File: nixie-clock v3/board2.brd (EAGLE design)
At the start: 158.4 x 50.2 mm, 15 parts

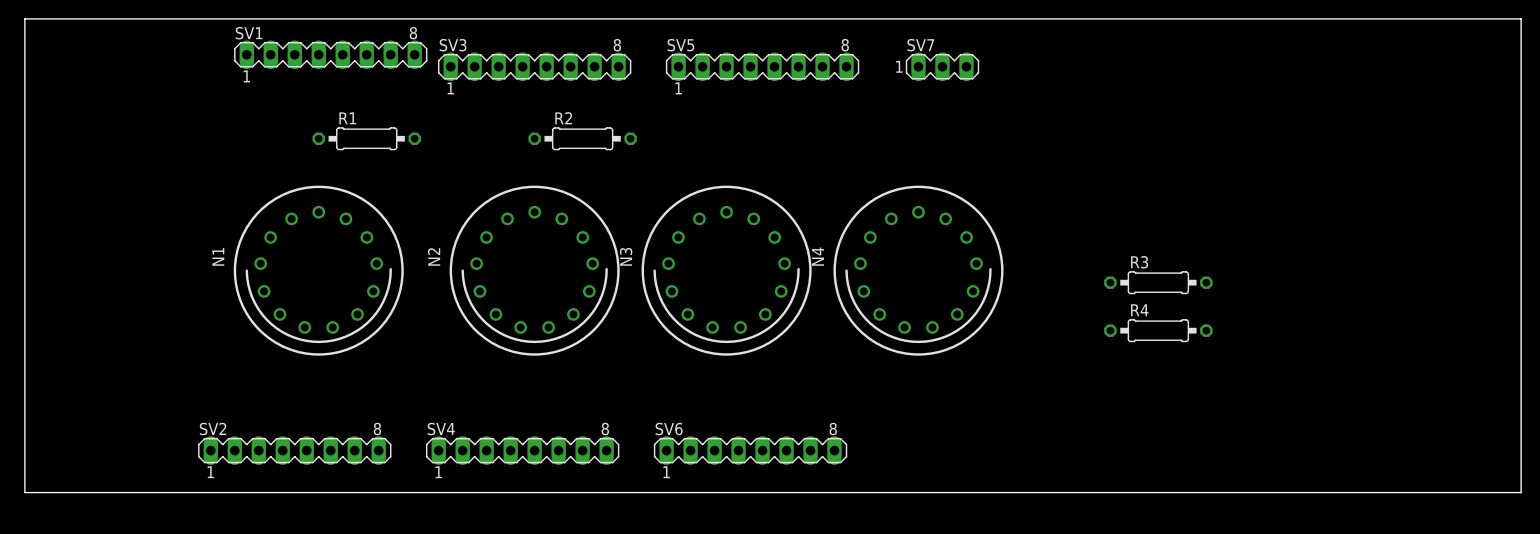
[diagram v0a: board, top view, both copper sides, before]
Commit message: lots of board progress
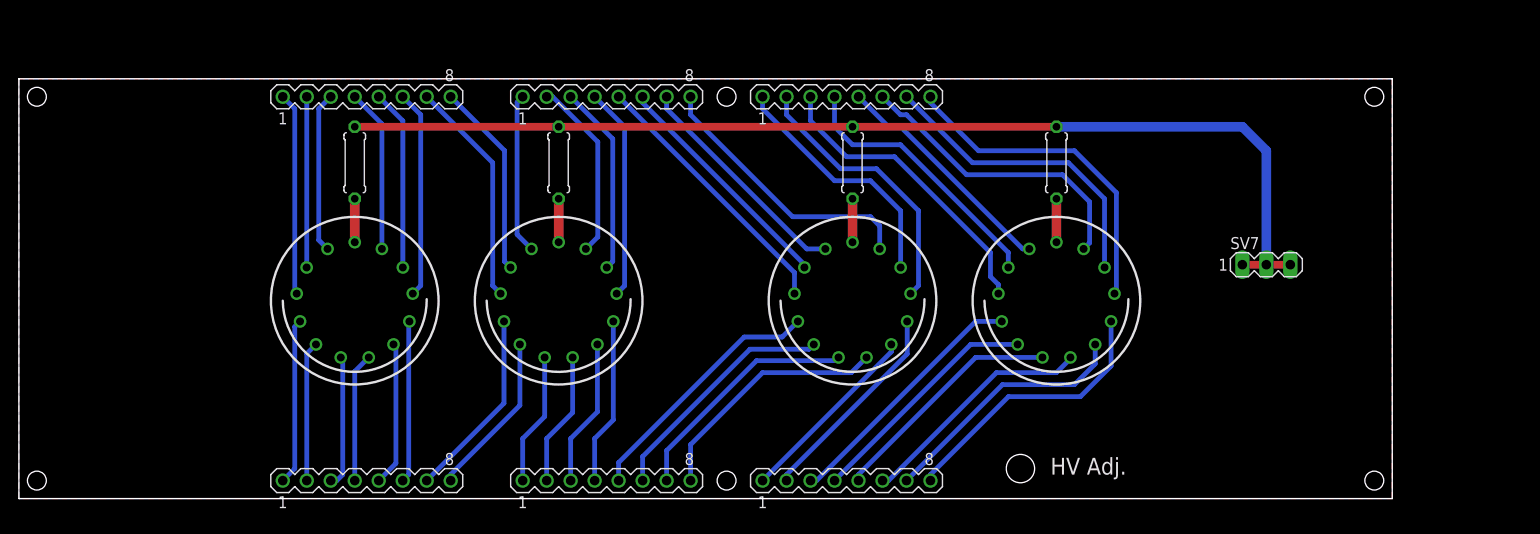
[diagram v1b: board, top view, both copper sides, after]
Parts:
- R1, R2, R3, R4: device resistor:0207/10 -> resistor:0207/7
- SV1, SV2, SV3, SV4, SV5, SV6: device con-lstb:MA08-1 -> con-lstb-mod:MA08-1
- moved SV7 40.2 mm to (132.1, 24.8)
- moved R3 34.8 mm to (88.3, 35.6), turned to 90 degrees
- moved R4 20.8 mm to (109.9, 35.6), turned to 90 degrees
- moved N4 14.9 mm to (109.9, 21.0)
- moved N3 13.7 mm to (88.3, 21.0)
- moved SV6 10.6 mm to (87.6, 1.91)
- moved SV5 9.44 mm to (87.6, 42.5)
- moved SV4 9.44 mm to (62.2, 1.91)
- moved SV2 8.25 mm to (36.8, 1.91)
- moved SV3 8.25 mm to (62.2, 42.5)
- moved SV1 5.85 mm to (36.8, 42.5)
- moved N1 4.96 mm to (35.6, 21.0)
- moved N2 4.07 mm to (57.1, 21.0)
- moved R2 3.59 mm to (57.1, 35.6), turned to 90 degrees
- moved R1 2.84 mm to (35.6, 35.6), turned to 90 degrees
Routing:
- net VCC/2: track 0.00 -> 114.7 mm
- net N4_2: track 0.00 -> 35.0 mm
- net N4_1: track 0.00 -> 32.7 mm
- net N4_9: track 0.00 -> 32.1 mm
- net N4_RHDP: track 0.00 -> 31.8 mm
- net N4_3: track 0.00 -> 29.2 mm
- net N3_RHDP: track 0.00 -> 29.2 mm
- net N3_2: track 0.00 -> 29.2 mm
- net N4_0: track 0.00 -> 28.7 mm
- net N3_9: track 0.00 -> 28.6 mm
- net N4_8: track 0.00 -> 27.2 mm
- net N4_4: track 0.00 -> 27.2 mm
- net N3_8: track 0.00 -> 27.1 mm
- net N3_1: track 0.00 -> 26.4 mm
- net N3_5: track 0.00 -> 26.3 mm
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- added copper zone on layer 16, net N$5
- added copper zone on layer 1, net N$6
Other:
- board size 158.4 x 50.2 mm -> 145.4 x 44.5 mm
- board text added: "HV Adj."
